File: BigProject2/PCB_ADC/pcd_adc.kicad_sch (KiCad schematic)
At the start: 19 parts, among them J1 I2C_input, J2 I2C_input, SW1 Mode_Calib, U1 ATmega328P-P, Y1 16MHz

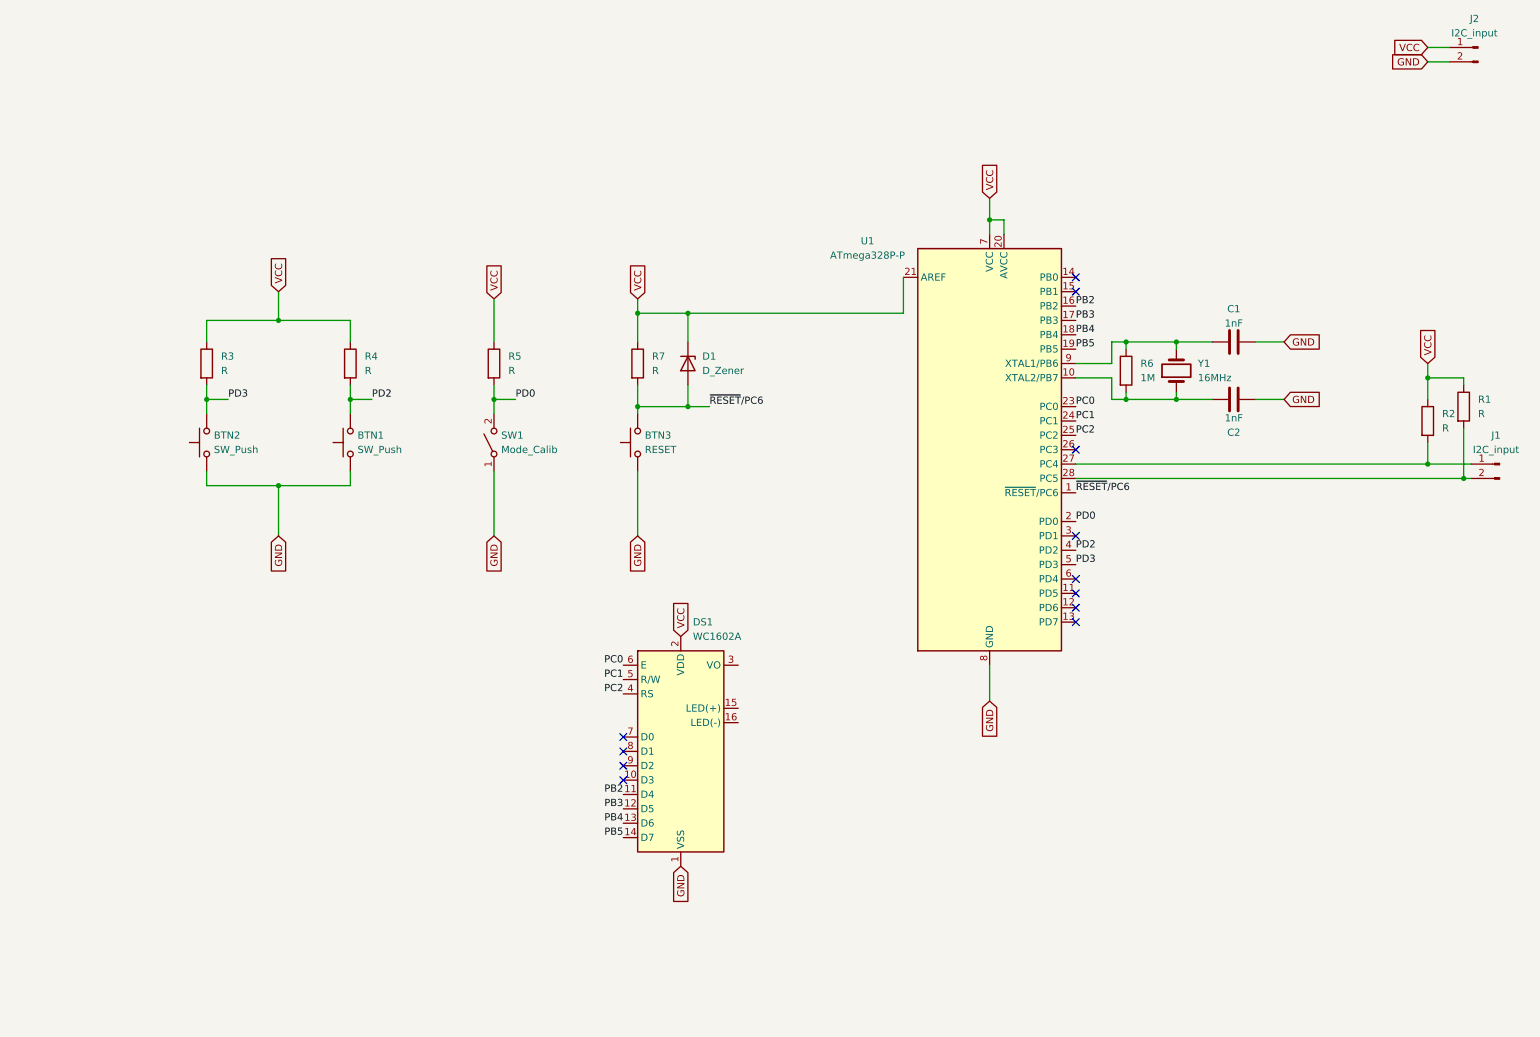
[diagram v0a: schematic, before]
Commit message: up
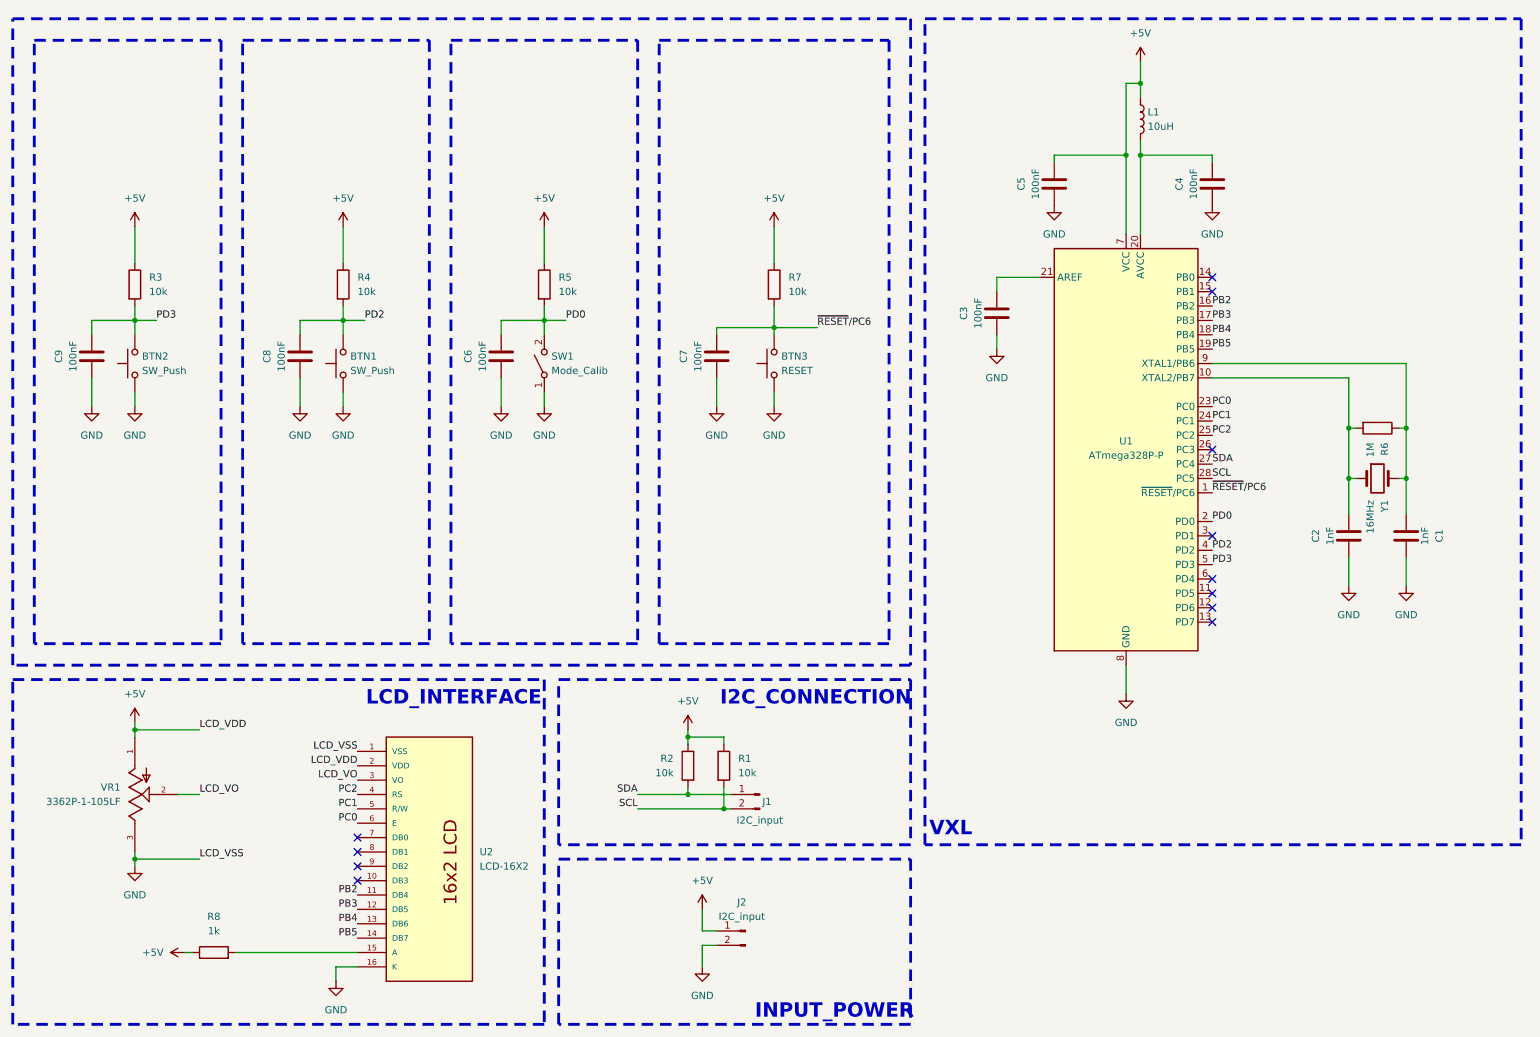
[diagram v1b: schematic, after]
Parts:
- removed D1: D_Zener, Diode_THT:D_DO-201AD_P15.24mm_Horizontal, symbol Device:D_Zener
- removed DS1: WC1602A, Display:WC1602A, symbol Display_Character:WC1602A
- added C3, C4, C5: 100nF, Capacitor_SMD:C_1206_3216Metric, symbol Device:C
- added C6, C7, C8, C9: 100nF, Capacitor_THT:C_Disc_D7.5mm_W5.0mm_P7.50mm, symbol Device:C
- added L1: 10uH, Inductor_SMD:L_1210_3225Metric, symbol Device:L
- added R8: 1k, Resistor_THT:R_Axial_DIN0207_L6.3mm_D2.5mm_P10.16mm_Horizontal, symbol Device:R
- added U2: LCD-16X2, LCD-16X2:MODULE_LCD-16X2, symbol LCD-16X2:LCD-16X2
- added VR1: 3362P-1-105LF, 3362W-1-105:TRIM_3362P-1-105LF, symbol 3362P-1-105LF:3362P-1-105LF
- BTN1, BTN2: footprint Button_Switch_THT:SW_PUSH_6mm -> Button_Switch_THT:SW_PUSH-12mm_Wuerth-430476085716
- C1, C2: footprint Capacitor_THT:CP_Radial_D10.0mm_P5.00mm -> Resistor_SMD:R_1206_3216Metric
- J1: footprint Connector_PinSocket_2.54mm:PinSocket_1x01_P2.54mm_Vertical -> Connector_PinHeader_2.54mm:PinHeader_1x02_P2.54mm_Horizontal
- J2: footprint Connector_PinSocket_2.54mm:PinSocket_1x01_P2.54mm_Vertical -> Connector_Samtec_HPM_THT:Samtec_HPM-02-05-x-S_Straight_1x02_Pitch5.08mm
- R1, R2, R3, R4, R5, R7: value R -> 10k; footprint Resistor_THT:R_Axial_DIN0918_L18.0mm_D9.0mm_P25.40mm_Horizontal -> Resistor_THT:R_Axial_DIN0207_L6.3mm_D2.5mm_P10.16mm_Horizontal
- R6: footprint Resistor_THT:R_Axial_DIN0918_L18.0mm_D9.0mm_P25.40mm_Horizontal -> Resistor_SMD:R_1206_3216Metric
- SW1: footprint Connector_PinHeader_2.54mm:PinHeader_1x02_P2.54mm_Vertical -> Button_Switch_SMD:SW_DIP_SPSTx01_Slide_Omron_A6S-110x_W8.9mm_P2.54mm
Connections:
- net GND: now also C3.1, C4.1, C5.1, C6.1, C7.1, C8.1, C9.1, U2.1 (VSS), U2.16 (K), VR1.3
- net PB2: now also U2.11 (DB4)
- net PB3: now also U2.12 (DB5)
- net PB4: now also U2.13 (DB6)
- net PB5: now also U2.14 (DB7)
- net PC0: now also U2.6 (E)
- net PC1: now also U2.5 (R/W)
- net PC2: now also U2.4 (RS)
- net PD0: now also C6.2
- net PD2: now also C8.2
- net PD3: now also C9.2
- net ~{RESET}/PC6: now also C7.2
- net SDA: now reaches J1.1 (Pin_1), R2.2, U1.27 (PC4)
- net SCL: now reaches J1.2 (Pin_2), R1.2, U1.28 (PC5)
- net VCC renamed +5V
- net +5V: now also C5.2, L1.1, R8.1, U2.2 (VDD), VR1.1; no longer U1.20 (AVCC), U1.21 (AREF)
- new net: C3.2, U1.21 (AREF)
- new net: R8.2, U2.15 (A)
- new net: C4.2, L1.2, U1.20 (AVCC)
- new net LCD_VO: U2.3 (VO), VR1.2
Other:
- note added: "I2C_CONNECTION"
- note added: "INPUT_POWER"
- note added: "LCD_INTERFACE"
- note added: "VXL"
- moved on the sheet: BTN1, BTN2, BTN3, C1, C2, J1, J2, R1, R2, R3, R4, R5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
